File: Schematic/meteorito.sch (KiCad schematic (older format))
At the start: 4 parts, among them P1 DH22, P2 GY-ML8511, P3 BMP180, U1 WeMos_mini

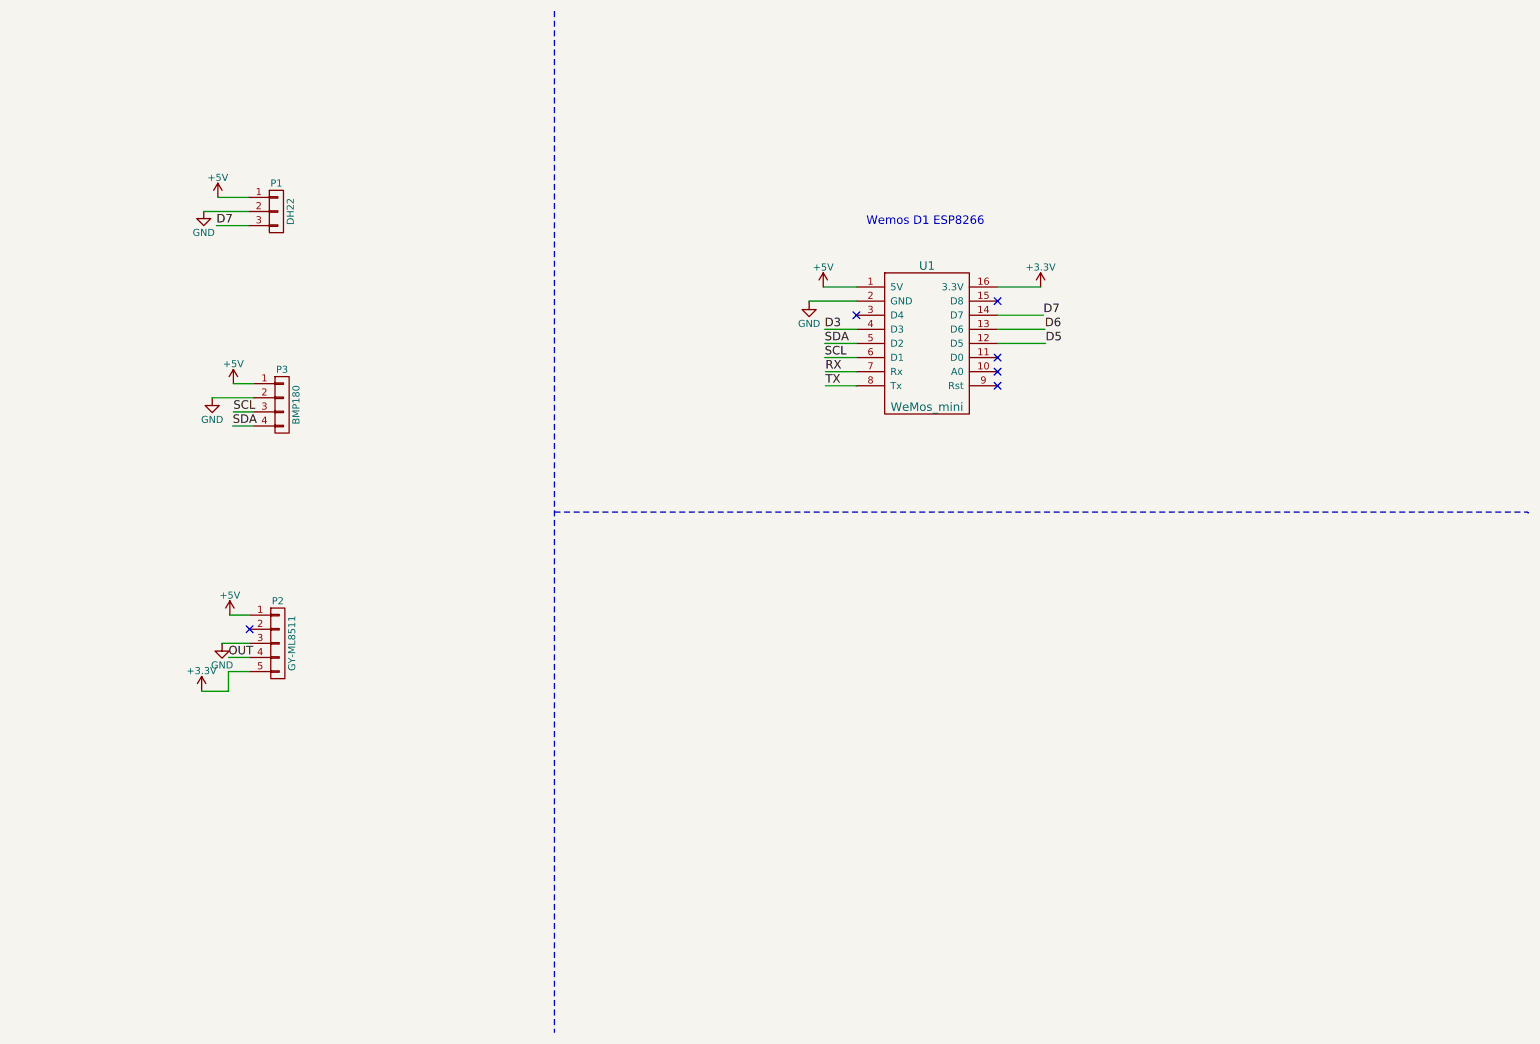
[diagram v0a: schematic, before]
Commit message: Update conectores
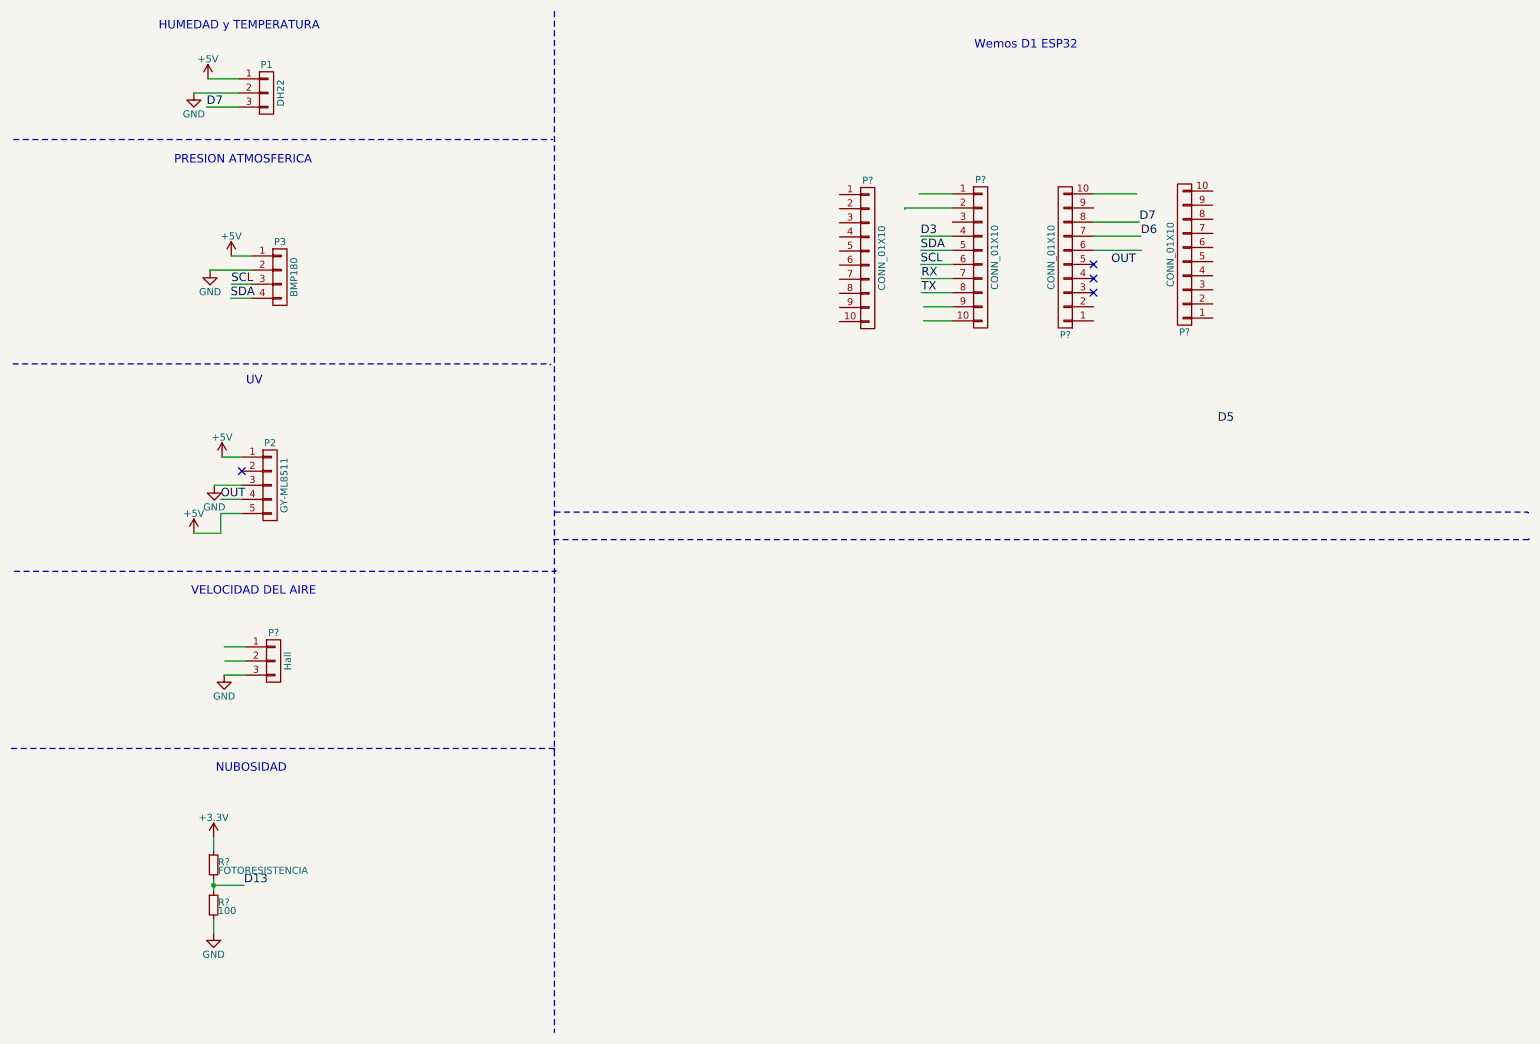
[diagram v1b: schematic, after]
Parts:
- removed U1: WeMos_mini, symbol WeMos_mini
- added P?: Hall, symbol CONN_01X03
- added P? (x4): CONN_01X10, symbol CONN_01X10
- added R?: FOTORESISTENCIA, symbol R_Small
- added R?: 100, symbol R_Small
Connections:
- net labels added: D13
- wire segments 27 -> 36
- no-connect marks 6 -> 4
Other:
- note added: "HUMEDAD y TEMPERATURA"
- note added: "NUBOSIDAD"
- note added: "PRESION ATMOSFERICA"
- note added: "UV"
- note added: "VELOCIDAD DEL AIRE"
- note added: "Wemos D1 ESP32"
- note removed: "Wemos D1 ESP8266"
- moved on the sheet: P1, P2, P3
